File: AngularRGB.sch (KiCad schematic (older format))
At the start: 4 parts

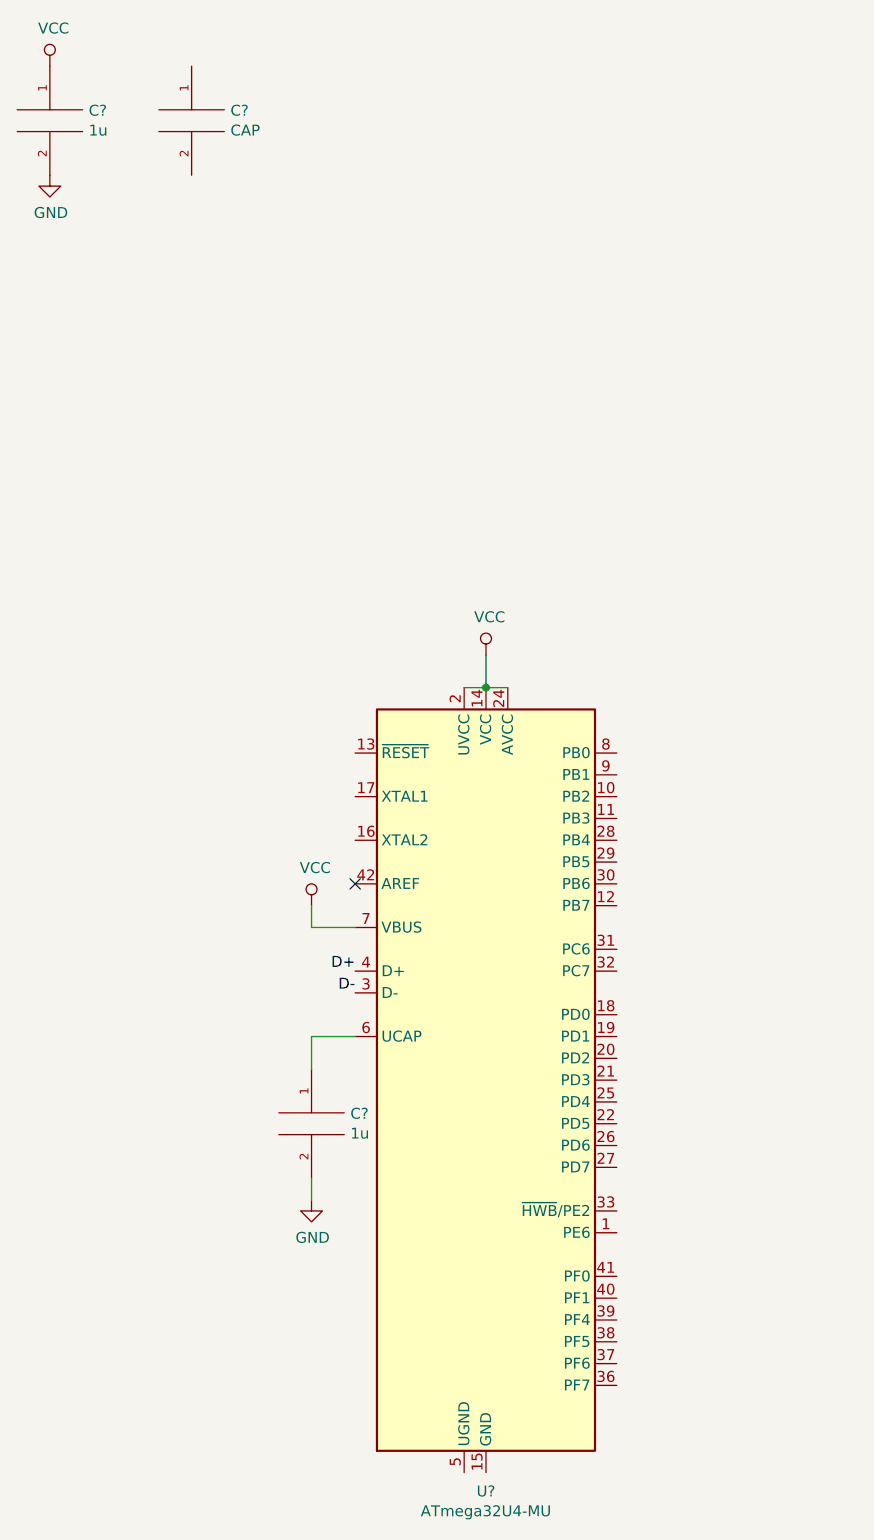
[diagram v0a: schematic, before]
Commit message: MCU Connections
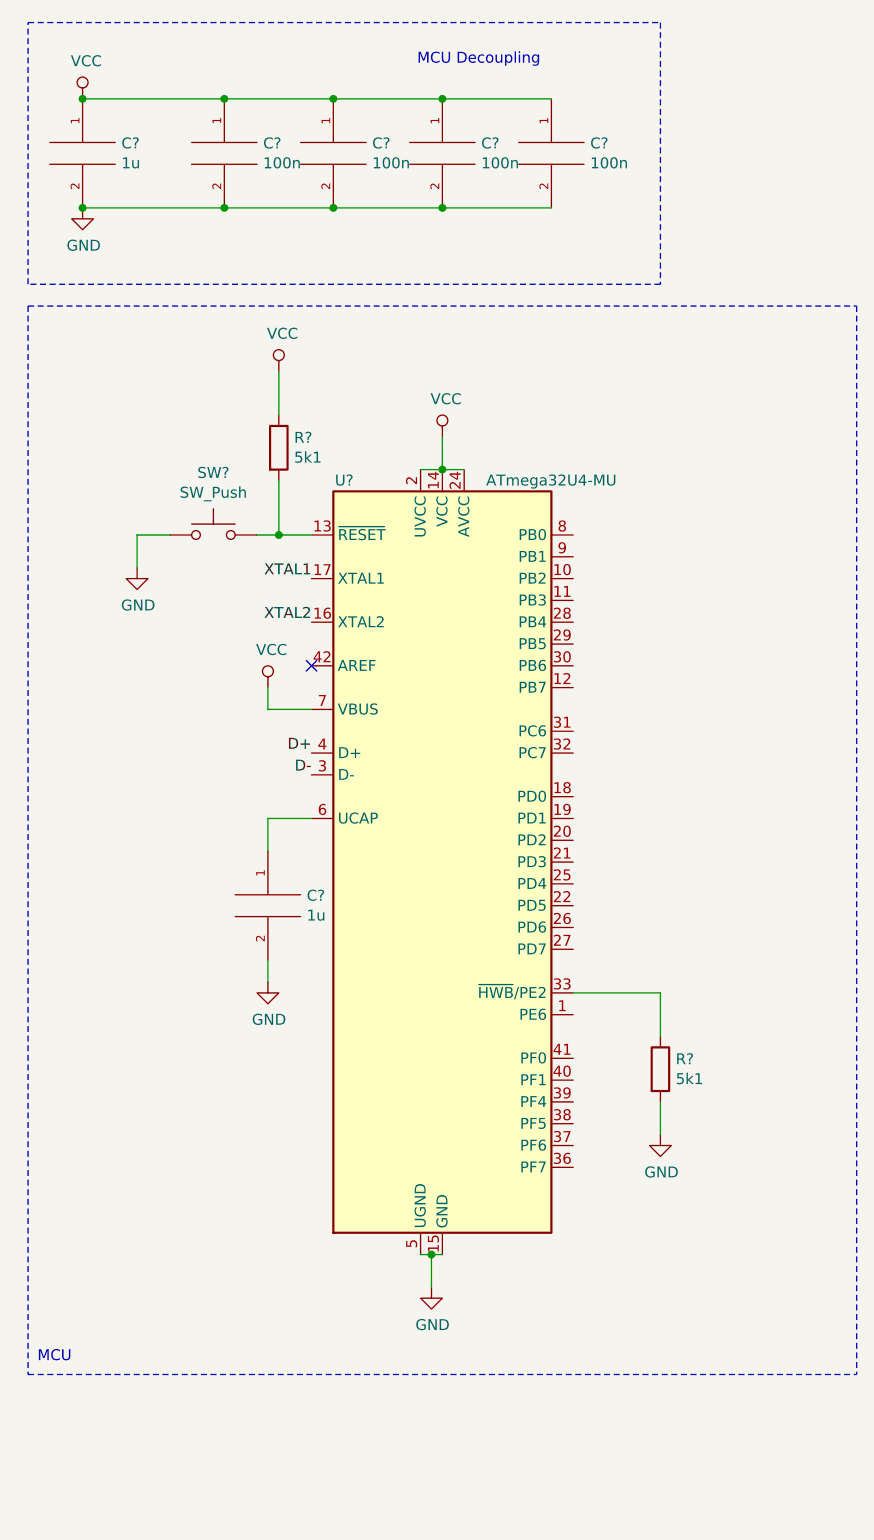
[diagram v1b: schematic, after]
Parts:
- added C? (x3): 100n, symbol pspice:CAP
- added R? (x2): 5k1, symbol Device:R
- added SW?: SW_Push, symbol Switch:SW_Push
- C?: value CAP -> 100n
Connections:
- net GND: now also C?.2, U?.15 (GND), U?.23 (GND), U?.35 (GND), U?.43 (GND), U?.45 (GND), U?.5 (UGND), C?.2, C?.2, C?.2, R?.2, SW?.1
- net VCC: now also C?.1, C?.1, C?.1, C?.1, R?.1
- net at U?.13 (~RESET): now also R?.2, SW?.2
- net XTAL2: now reaches U?.16 (XTAL2)
- net XTAL1: now reaches U?.17 (XTAL1)
- net at U?.33 (~HWB~/PE2): now also R?.1
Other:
- note added: "MCU Decoupling"
- note added: "MCU\n"
- moved on the sheet: C?, U?
